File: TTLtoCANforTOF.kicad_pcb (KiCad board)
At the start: 2 copper layers, 36 x 20.1 mm, 43 parts, among them J2 CAN, J3 TOF, J4 XT30, J6 SWD, Q2 Si2309CDS-T1-GE3, SW1 SW_SPST, U1 TPS54202DDC, U2 ME6211C33M5, U3 STM32G0B1CBTx, U6 TCAN3413DR, Y1 X32258MSB

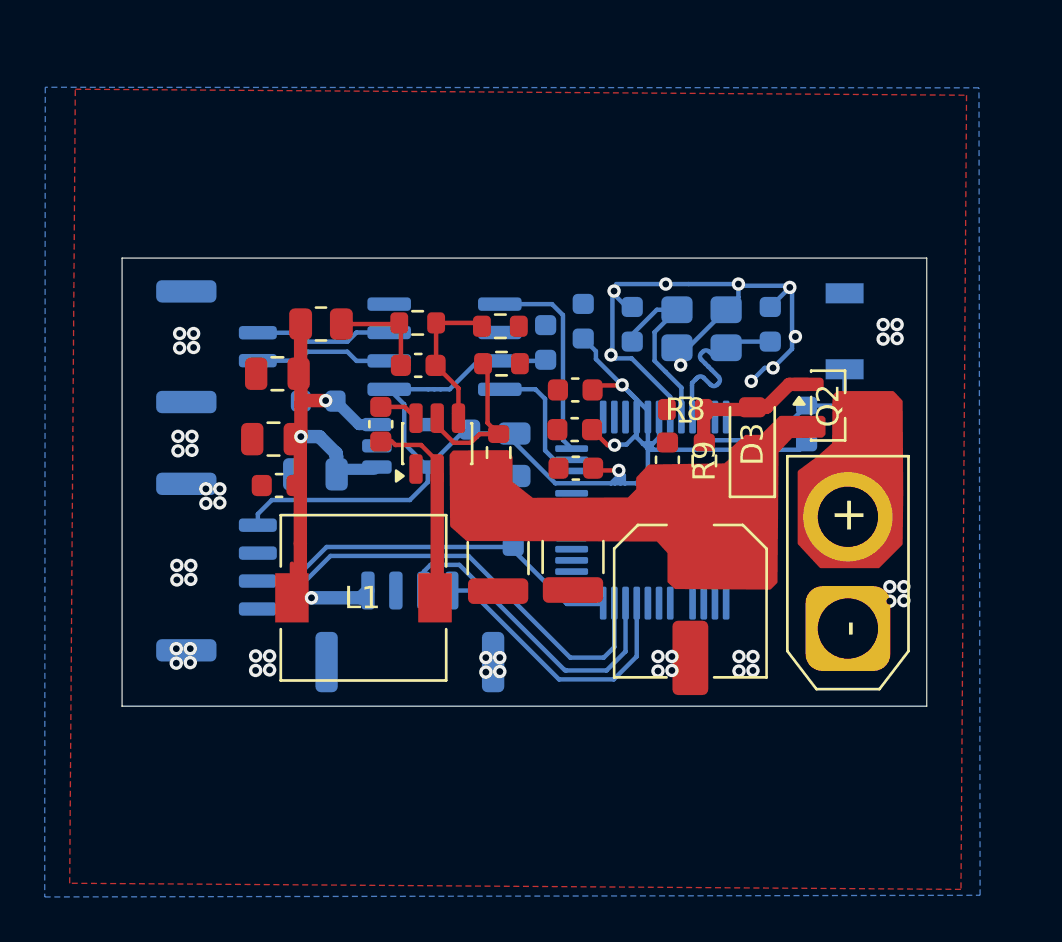
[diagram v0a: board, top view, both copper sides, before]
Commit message: 1
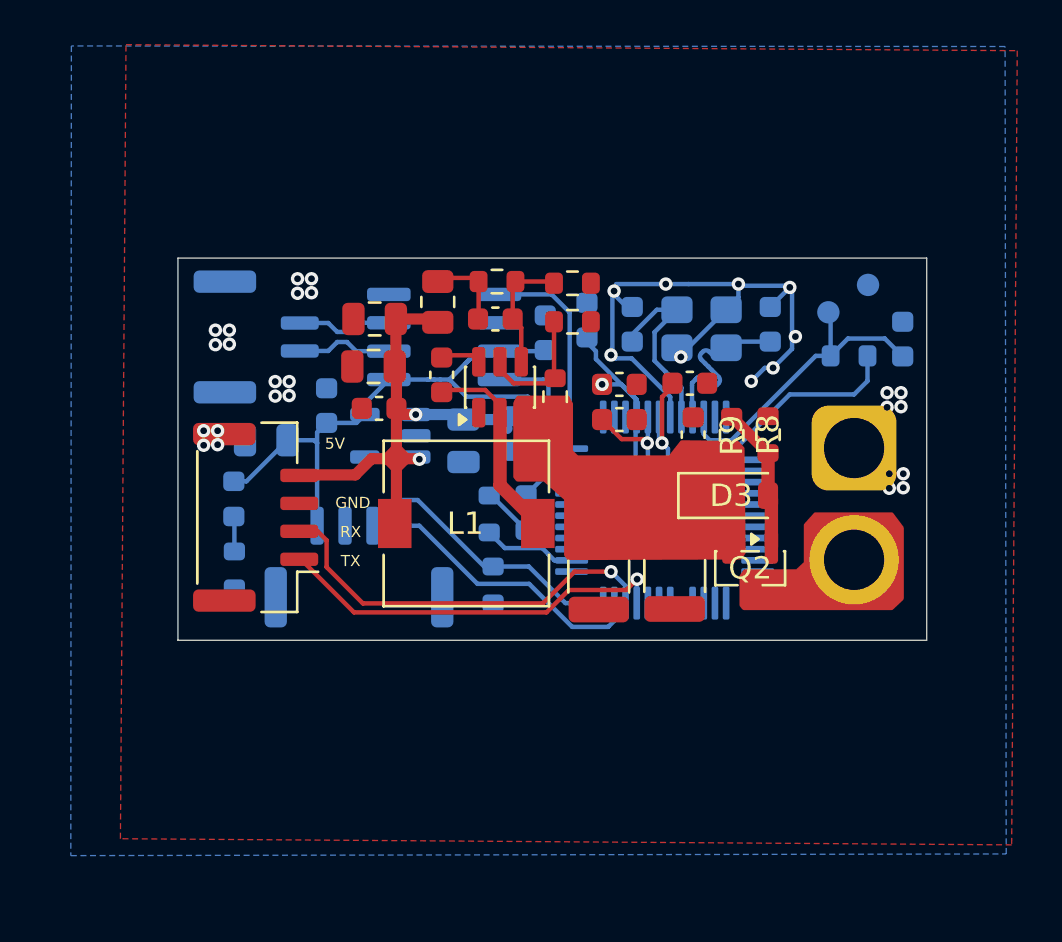
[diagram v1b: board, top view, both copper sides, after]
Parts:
- removed C22: 47uF, Capacitor_SMD:C_Elec_6.3x7.7
- removed SW1: SW_SPST, Button_Switch_SMD:SW_SPST_B3U-1000P
- added D1: LED, LED_SMD:LED_0603_1608Metric, B.Cu at (153.0, 71.2)
- added D2: LED, LED_SMD:LED_0603_1608Metric, B.Cu at (166.1, 71.8)
- added R10: 1kΩ, Resistor_SMD:R_0603_1608Metric, B.Cu at (153.0, 74.3)
- added R11: 1kΩ, Resistor_SMD:R_0603_1608Metric, B.Cu at (164.4, 71.8)
- added TP1: RST, TestPoint:TestPoint_Pad_D1.0mm, B.Cu at (179.6, 62.8)
- added TP2: GND, TestPoint:TestPoint_Pad_D1.0mm, B.Cu at (181.4, 61.6)
- J2: footprint Connector_JST:JST_GH_SM02B-GHS-TB_1x02-1MP_P1.25mm_Horizontal -> Connector_JST:JST_GH_BM02B-GHS-TBT_1x02-1MP_P1.25mm_Vertical
- J3: footprint Connector_JST:JST_GH_SM04B-GHS-TB_1x04-1MP_P1.25mm_Horizontal -> Connector_JST:JST_GH_BM04B-GHS-TBT_1x04-1MP_P1.25mm_Vertical; moved to F.Cu
- J4: moved to B.Cu
- moved C11 11.1 mm to (154.4, 68.5), turned to 180 degrees
- moved C10 8.70 mm to (165.3, 68.2), turned to -90 degrees
- moved J3 8.60 mm to (154.0, 72.0), turned to 90 degrees
- moved J4 8.08 mm to (180.8, 68.9), turned to -90 degrees
- moved Q2 8.07 mm to (176.1, 74.3), turned to -90 degrees
- moved C3 7.94 mm to (172.7, 74.6)
- moved C9 6.79 mm to (163.3, 68.6), turned to -90 degrees
- moved C12 6.66 mm to (157.2, 67.0), turned to 90 degrees
- moved J6 6.38 mm to (158.6, 74.2), turned to 180 degrees
- moved L1 5.68 mm to (163.4, 72.3)
- moved C20 5.65 mm to (159.5, 67.1)
- moved C8 5.53 mm to (159.2, 65.2)
- moved R3 5.32 mm to (162.1, 62.4), turned to 90 degrees
- moved C15 5.13 mm to (173.4, 66.0), turned to 0 degrees
- moved C6 4.99 mm to (159.3, 63.1)
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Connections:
- J2 pad 1: /CAN- -> /CAN+
- J2 pad 2: /CAN+ -> /CAN-
- U3 pad 38: unconnected-(U3-PD0-Pad38) -> /LED
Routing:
- net +3.3V: track 60.8 -> 70.3 mm
- net /SWDIO: track 21.0 -> 12.3 mm
- net /USART1_TX: track 12.7 -> 17.8 mm, vias 0 -> 1
- net /NRST: track 9.52 -> 14.0 mm
- net /SWCLK: track 17.2 -> 12.8 mm
- net /LED: track 0.00 -> 4.21 mm
- net /USART1_RX: track 14.5 -> 18.3 mm, vias 0 -> 1
- net Net-(D2-K): track 0.00 -> 2.29 mm
- net Net-(D1-K): track 0.00 -> 1.57 mm
- net Net-(U1-FB): track 6.99 -> 5.56 mm
- net /CAN+: track 5.66 -> 4.32 mm
- net /CAN-: track 5.66 -> 4.32 mm
- net Net-(U1-EN): track 7.01 -> 5.71 mm
- net Net-(U1-SW): track 8.37 -> 9.25 mm
- net Net-(C7-Pad1): track 4.41 -> 3.58 mm
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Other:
- board size 36 x 20.1 mm -> 33.5 x 17.1 mm
